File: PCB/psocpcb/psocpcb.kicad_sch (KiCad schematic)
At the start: 24 parts, among them J1 Conn_01x04_Pin, J2 Conn_01x06_Pin, J3 Conn_01x04_Pin, J4 Conn_01x07_Pin, U1 CYBLE-416045-02

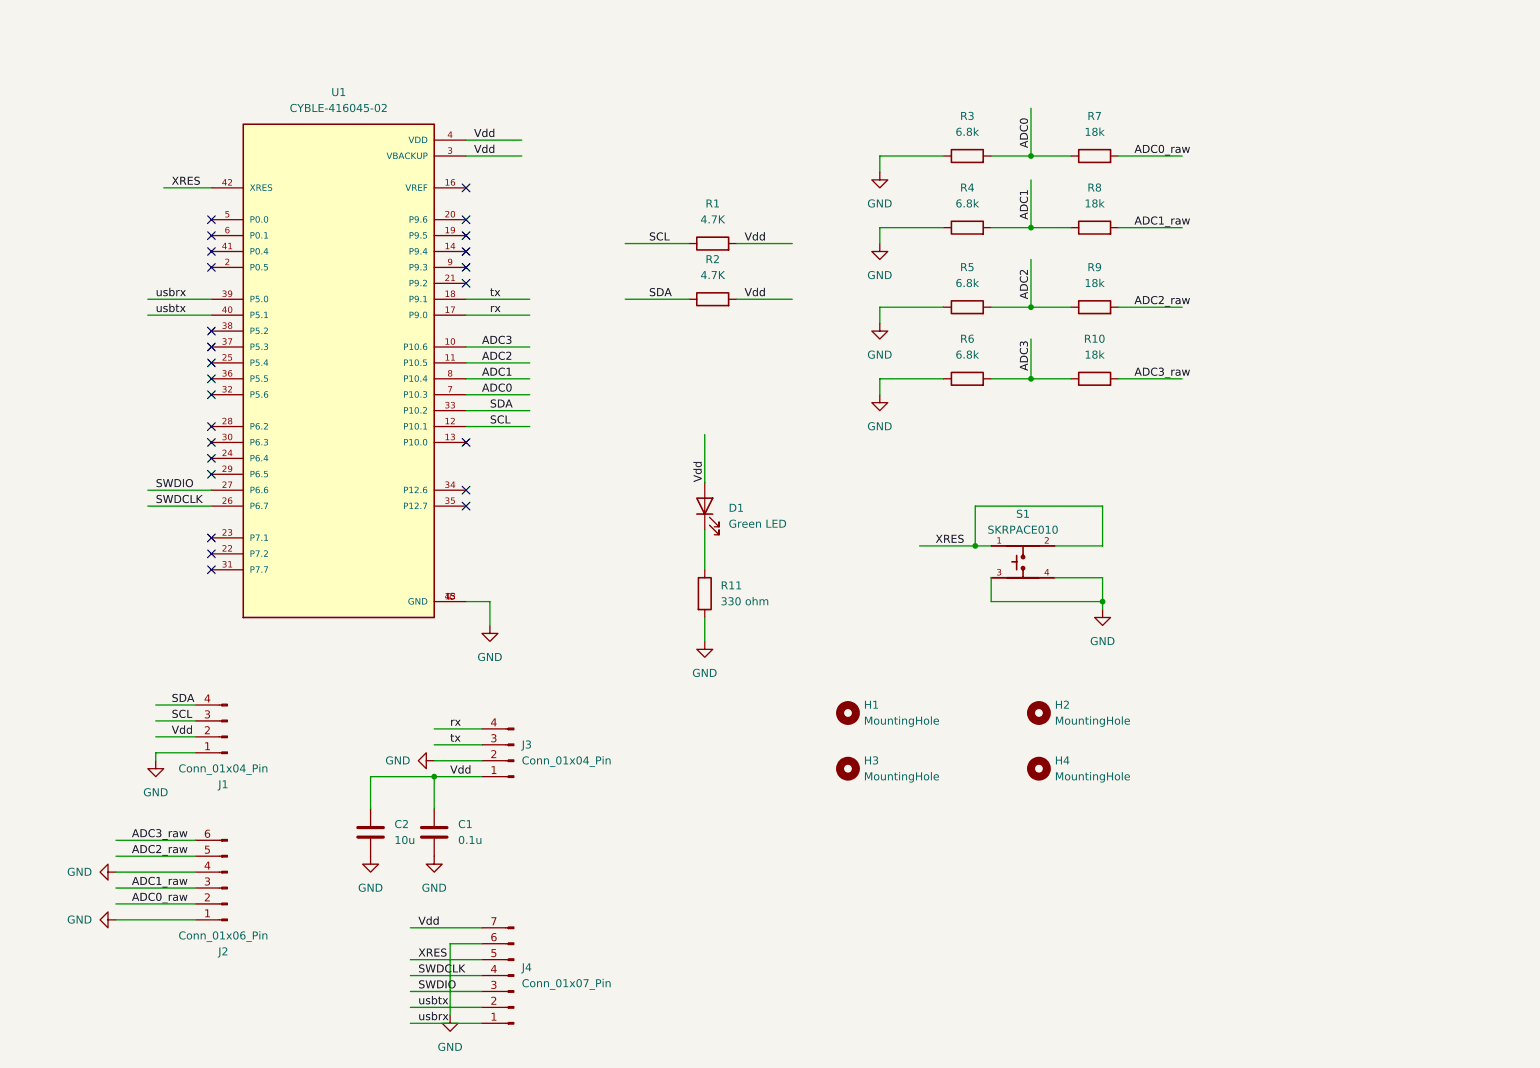
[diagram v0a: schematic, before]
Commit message: second review
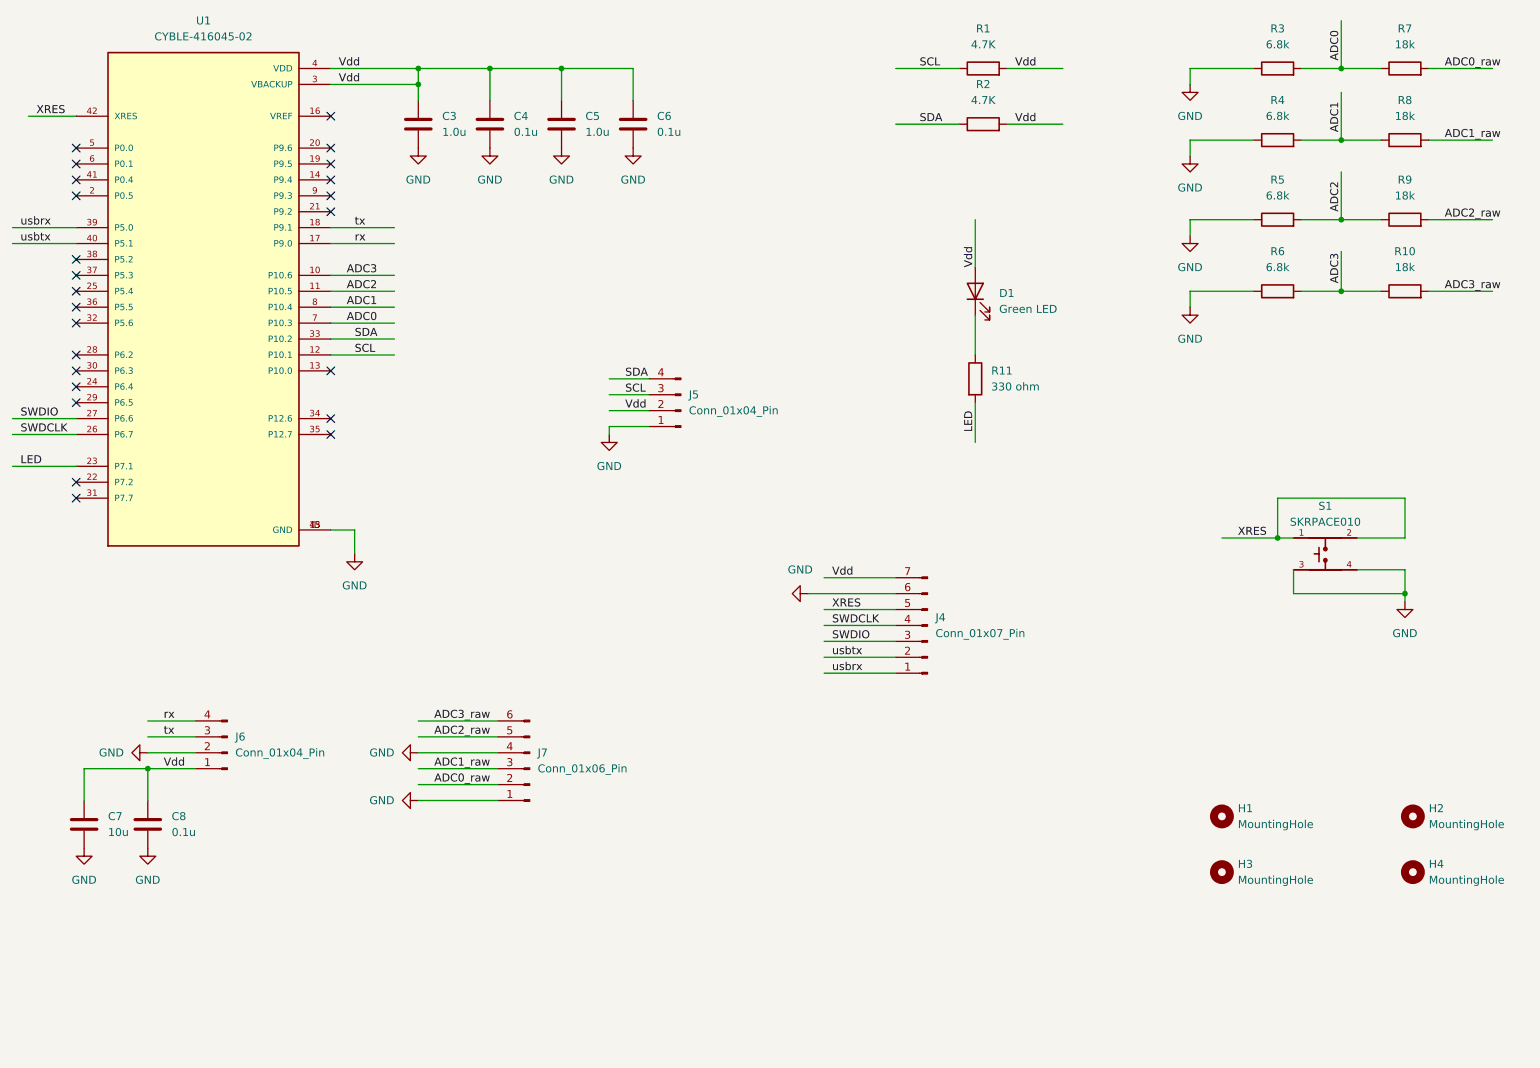
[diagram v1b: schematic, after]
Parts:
- removed C1: 0.1u, Capacitor_SMD:C_0603_1608Metric, symbol Device:C
- removed C2: 10u, Capacitor_SMD:C_0603_1608Metric, symbol Device:C
- removed J1, J3: Conn_01x04_Pin, Connector_PinHeader_2.54mm:PinHeader_1x04_P2.54mm_Vertical, symbol Connector:Conn_01x04_Pin
- removed J2: Conn_01x06_Pin, Connector_PinHeader_2.54mm:PinHeader_1x06_P2.54mm_Vertical, symbol Connector:Conn_01x06_Pin
- added C3, C5: 1.0u, Capacitor_SMD:C_0603_1608Metric, symbol Device:C
- added C4, C6, C8: 0.1u, Capacitor_SMD:C_0603_1608Metric, symbol Device:C
- added C7: 10u, Capacitor_SMD:C_0603_1608Metric, symbol Device:C
- added J5, J6: Conn_01x04_Pin, Connector_JST:JST_PH_S4B-PH-K_1x04_P2.00mm_Horizontal, symbol Connector:Conn_01x04_Pin
- added J7: Conn_01x06_Pin, Connector_JST:JST_PH_S6B-PH-K_1x06_P2.00mm_Horizontal, symbol Connector:Conn_01x06_Pin
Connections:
- net ADC0_raw: now also J7.2 (Pin_2)
- net ADC1_raw: now also J7.3 (Pin_3)
- net ADC2_raw: now also J7.5 (Pin_5)
- net ADC3_raw: now also J7.6 (Pin_6)
- net GND: now also C3.2, C4.2, C5.2, C6.2, C7.2, C8.2, J5.1 (Pin_1), J6.2 (Pin_2), J7.1 (Pin_1), J7.4 (Pin_4); no longer R11.2
- net SCL: now also J5.3 (Pin_3)
- net SDA: now also J5.4 (Pin_4)
- net Vdd: now also C3.1, C4.1, C5.1, C6.1, C7.1, C8.1, J5.2 (Pin_2), J6.1 (Pin_1)
- net rx: now also J6.4 (Pin_4)
- net tx: now also J6.3 (Pin_3)
- net LED: now reaches U1.23 (P7.1)
- net LED: now also R11.2
- no-connect marks 25 -> 24
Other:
- moved on the sheet: D1, H1, H2, H3, H4, J4, R1, R10, R11, R2, R3, R4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
